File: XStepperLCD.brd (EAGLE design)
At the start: 49.5 x 38.1 mm, 38 parts, among them U1 LCD-16X2NOHOLES, X1 RJ45-6L-B

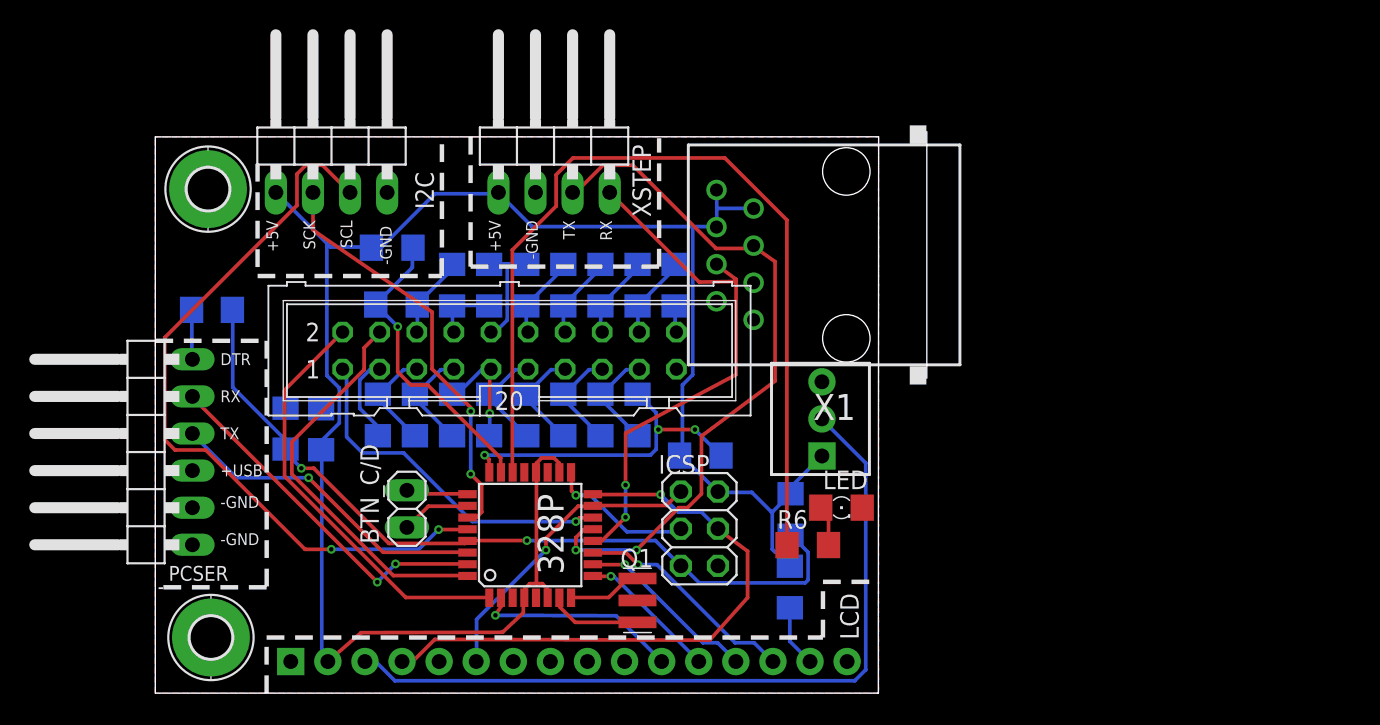
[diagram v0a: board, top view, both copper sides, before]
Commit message: make board bigger
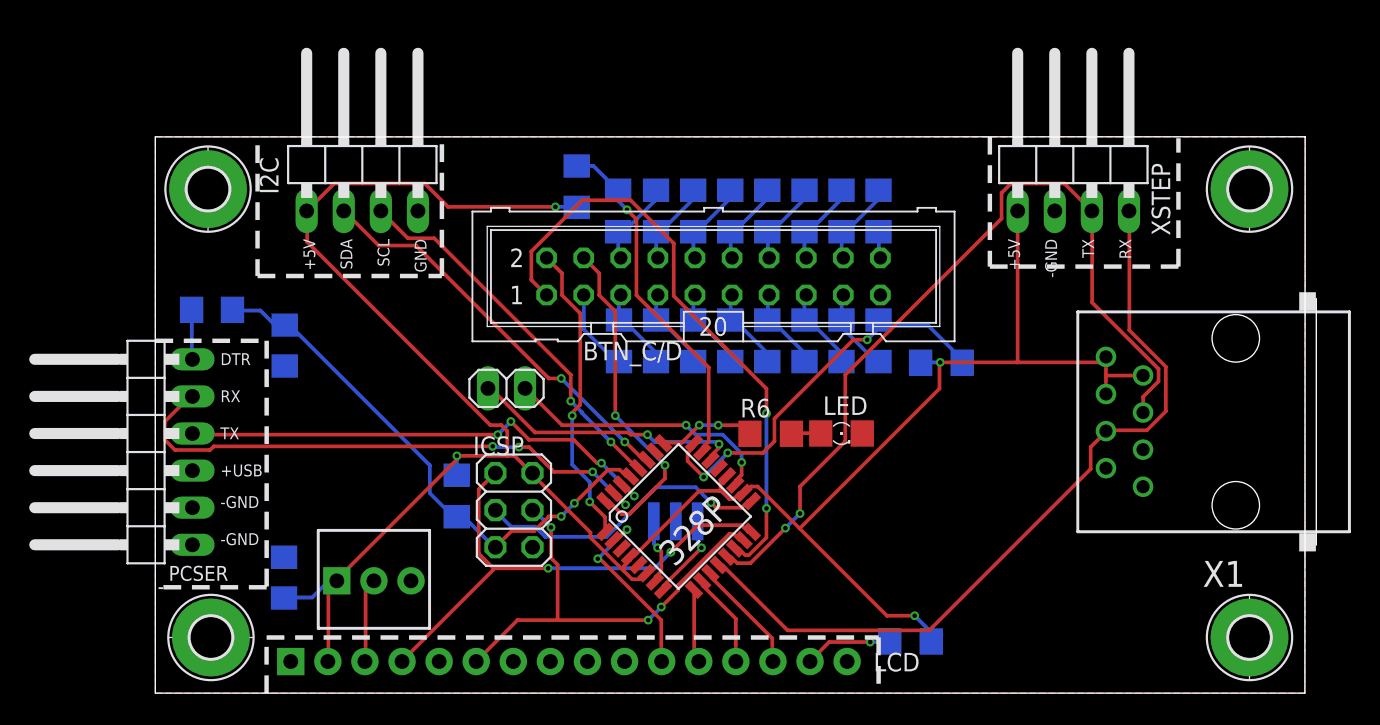
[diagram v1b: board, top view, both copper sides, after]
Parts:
- added H1, H2: MOUNT-PAD-ROUND2.8, holes:2,8-PAD
- moved XSTEP 35.6 mm to (62.9, 36.8)
- moved R1 32.2 mm to (15.0, 8.00), turned to 0 degrees
- moved X1 29.0 mm to (74.0, 18.6)
- moved R3 22.9 mm to (20.6, 13.5)
- moved R4 17.7 mm to (53.8, 22.6)
- moved R16 17.3 mm to (49.5, 24.1)
- moved R17 17.3 mm to (47.0, 24.1)
- moved R18 17.3 mm to (44.5, 24.1)
- moved R19 17.3 mm to (41.9, 24.1)
- moved R20 17.3 mm to (39.4, 24.1)
- moved R21 17.3 mm to (36.8, 24.1)
- moved R22 17.3 mm to (34.3, 24.1)
- moved R23 17.3 mm to (31.8, 24.1)
- moved R8 16.5 mm to (31.7, 33.0), turned to 90 degrees
- moved BUTTONS 14.9 mm to (38.2, 28.5)
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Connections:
- net BUTTONS_C: now also 328P.19; no longer 328P.25
- net BUTTONS_D: now also 328P.22; no longer 328P.26
- net ENABLE/MOSI: now also ICSP.4; no longer ICSP.1
- net N$15: now also 328P.25; no longer 328P.22
- net RS/MISO: now also ICSP.1; no longer ICSP.4
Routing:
- net N$15: track 61.9 -> 6.72 mm, vias 0 -> 2
- net N$1: track 53.6 -> 5.78 mm
- net SCL: track 51.0 -> 26.0 mm
- net VCC: track 132.2 -> 156.9 mm, vias 0 -> 4
- net RX: track 36.7 -> 54.4 mm, vias 2 -> 0
- net POT_SELECT: track 24.1 -> 41.4 mm, vias 1 -> 2
- net RESET: track 54.5 -> 37.5 mm
- net BUTTONS_C: track 4.26 -> 19.0 mm, vias 0 -> 2
- net BUTTONS_D: track 4.76 -> 18.7 mm, vias 0 -> 2
- net USB_RXD: track 24.7 -> 38.6 mm, vias 2 -> 4
- net USB_TXD: track 22.2 -> 34.0 mm, vias 1 -> 4
- net SCK: track 10.0 -> 20.6 mm
- net ENABLE/MOSI: track 21.0 -> 30.6 mm, vias 1 -> 3
- net TX: track 48.3 -> 57.6 mm
- net POT_B: track 29.0 -> 20.9 mm, vias 0 -> 2
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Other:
- board size 49.5 x 38.1 mm -> 78.7 x 38.1 mm
- board text added: "GND"
- board text added: "SDA"
- board text removed: "SCK"
